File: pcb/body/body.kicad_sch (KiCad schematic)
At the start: 3 parts, among them J1 Conn_01x08_Socket, J2 Conn_01x05_Pin, U1 Teensy4.1

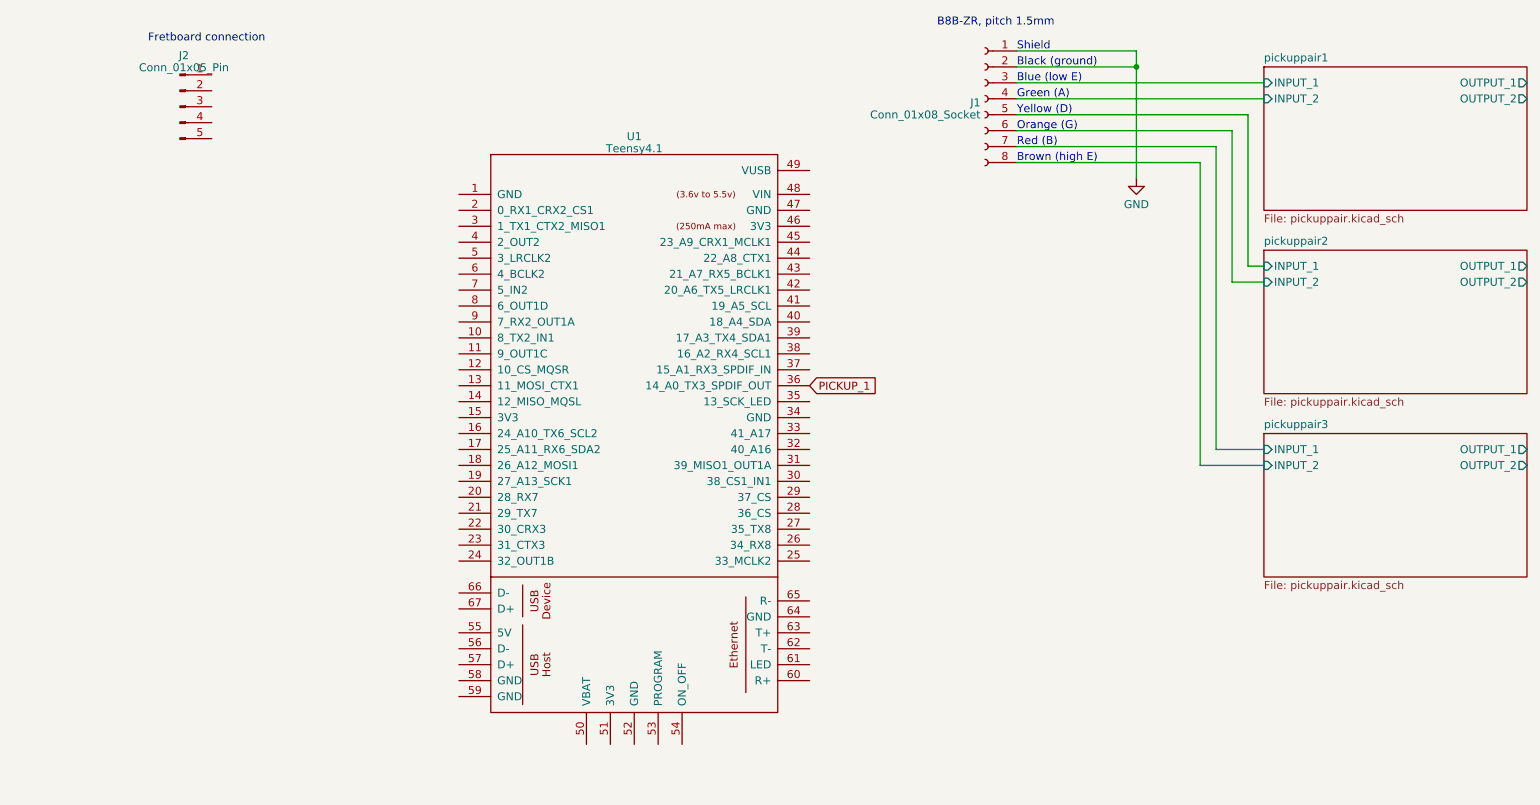
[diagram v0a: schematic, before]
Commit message: output stage
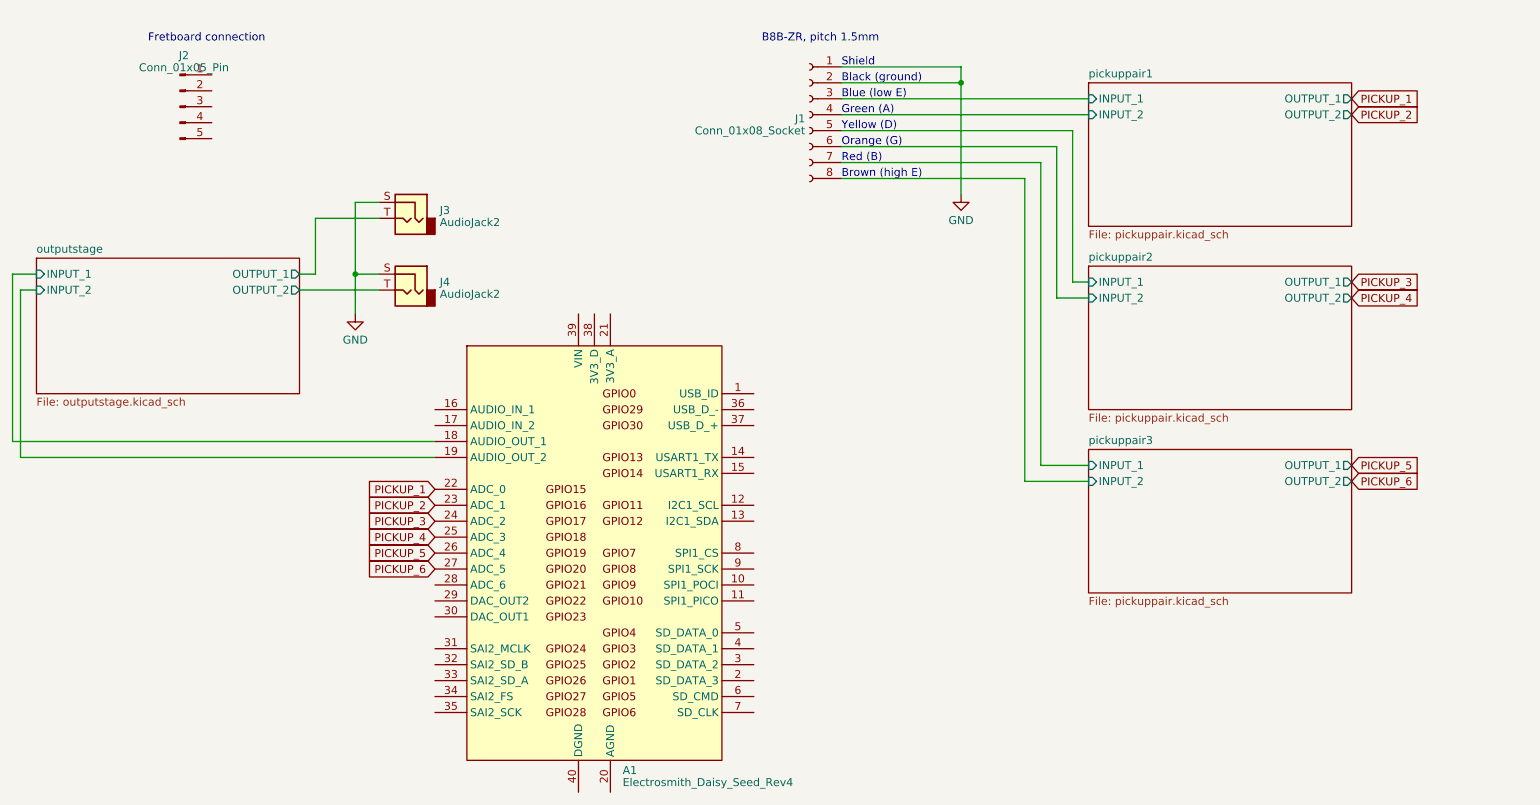
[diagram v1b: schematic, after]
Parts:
- removed U1: Teensy4.1, symbol teensy:Teensy4.1
- added A1: Electrosmith_Daisy_Seed_Rev4, Module:Electrosmith_Daisy_Seed, symbol MCU_Module:Electrosmith_Daisy_Seed_Rev4
- added J3, J4: AudioJack2, symbol Connector_Audio:AudioJack2
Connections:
- net GND: now also J3.S, J4.S
- net PICKUP_1: now also A1.22 (ADC_0)
- new net PICKUP_2: A1.23 (ADC_1)
- new net PICKUP_3: A1.24 (ADC_2)
- new net PICKUP_4: A1.25 (ADC_3)
- new net PICKUP_5: A1.26 (ADC_4)
- new net PICKUP_6: A1.27 (ADC_5)
- new net outputstage/INPUT_1: A1.18 (AUDIO_OUT_1)
- new net outputstage/INPUT_2: A1.19 (AUDIO_OUT_2)
- new net outputstage/OUTPUT_1: J3.T
- new net outputstage/OUTPUT_2: J4.T
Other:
- added sheet outputstage (outputstage.kicad_sch)
- moved on the sheet: J1
